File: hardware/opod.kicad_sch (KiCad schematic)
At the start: 1 part, among them U1 STM32F411CEUx

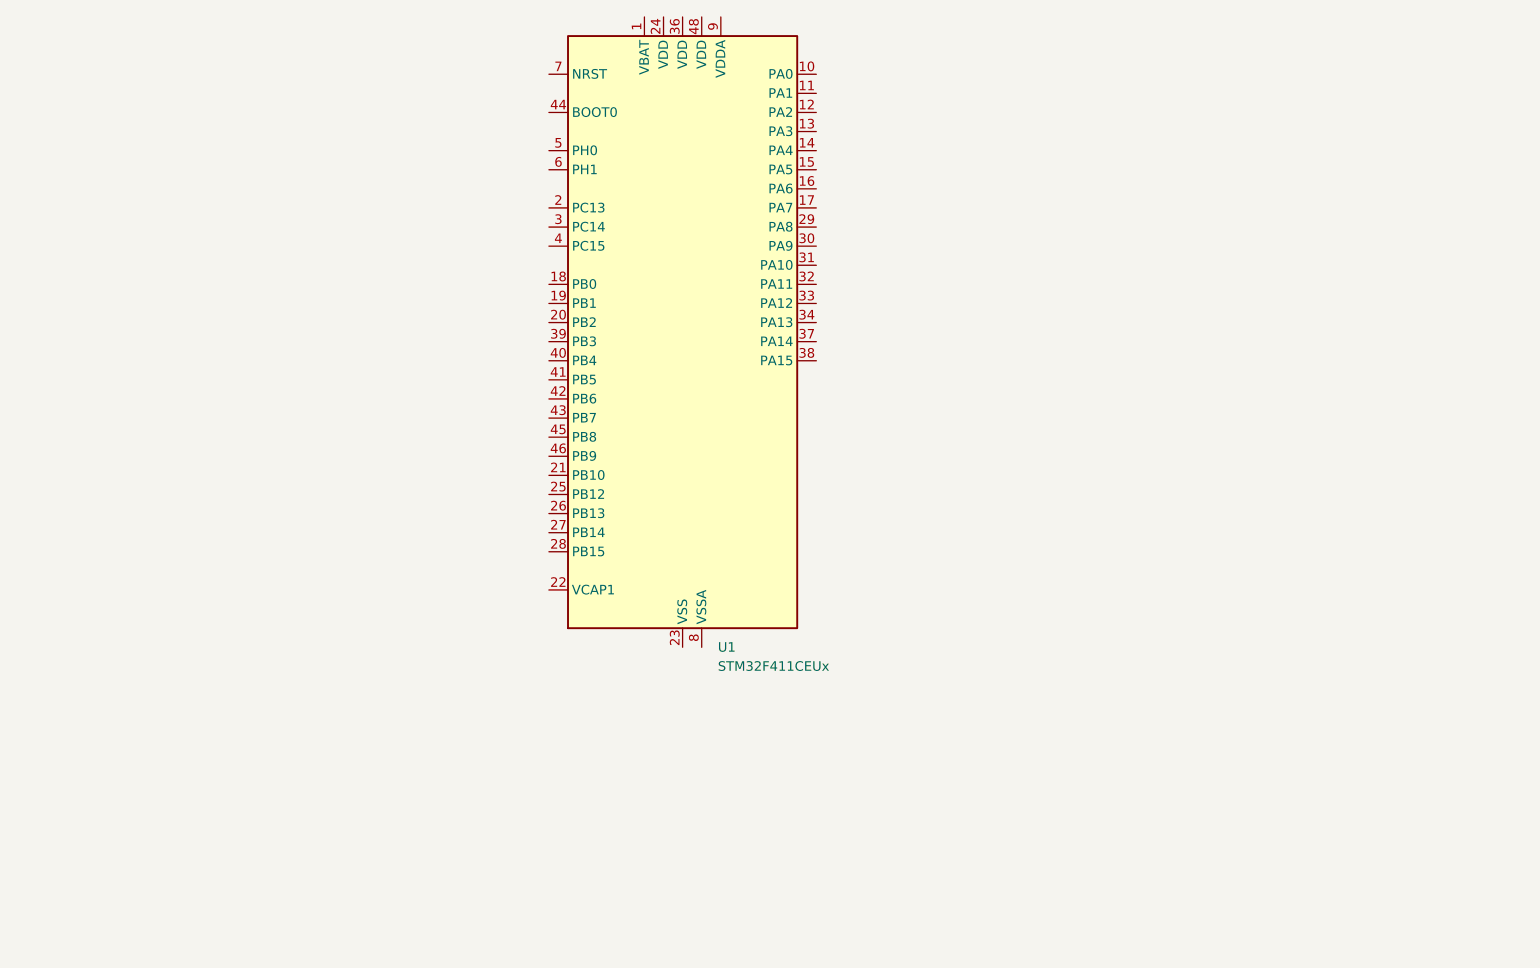
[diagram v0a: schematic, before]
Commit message: Hello, World x2
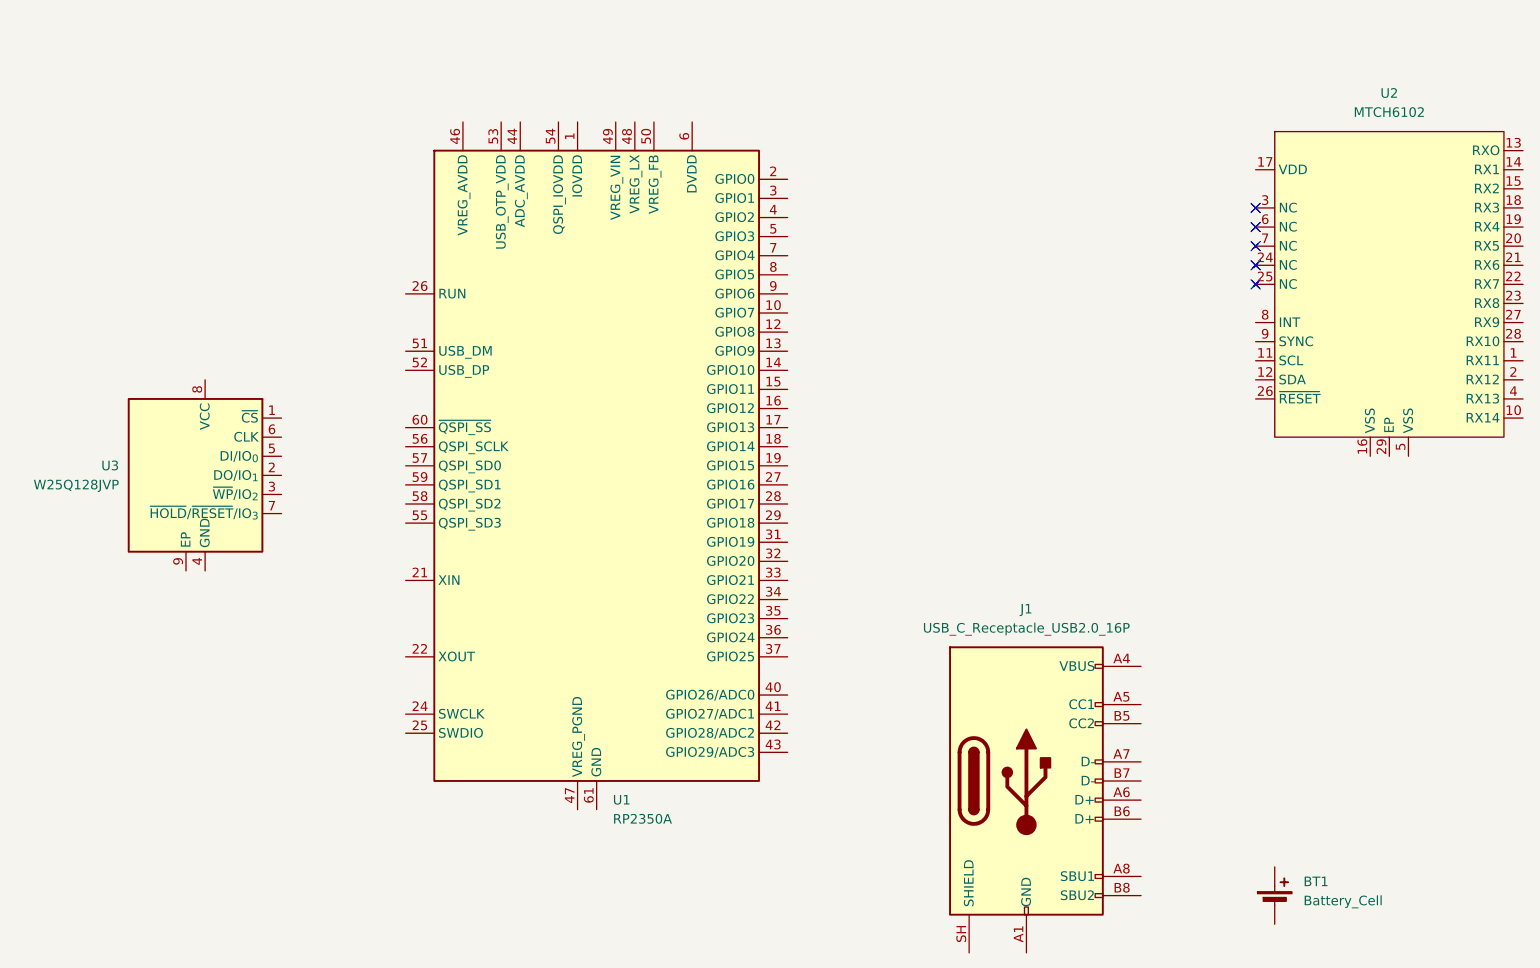
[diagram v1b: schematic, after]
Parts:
- removed U1: STM32F411CEUx, Package_DFN_QFN:QFN-48-1EP_7x7mm_P0.5mm_EP5.6x5.6mm, symbol MCU_ST_STM32F4:STM32F411CEUx
- added BT1: Battery_Cell, symbol Device:Battery_Cell
- added J1: USB_C_Receptacle_USB2.0_16P, symbol Connector:USB_C_Receptacle_USB2.0_16P
- added U1: RP2350A, Package_DFN_QFN:QFN-60-1EP_7x7mm_P0.4mm_EP3.4x3.4mm, symbol MCU_RaspberryPi:RP2350A
- added U2: MTCH6102, Package_DFN_QFN:UQFN-28-1EP_4x4mm_P0.4mm_EP2.35x2.35mm, symbol Sensor_Touch:MTCH6102-I/MV
- added U3: W25Q128JVP, Package_SON:WSON-8-1EP_6x5mm_P1.27mm_EP3.4x4.3mm, symbol Memory_Flash:W25Q128JVP
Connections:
- new net: U1.1 (IOVDD), U1.11 (IOVDD), U1.20 (IOVDD), U1.30 (IOVDD), U1.38 (IOVDD), U1.45 (IOVDD)
- new net: U1.23 (DVDD), U1.39 (DVDD), U1.6 (DVDD)
- new net: J1.A1 (GND), J1.A12 (GND), J1.B1 (GND), J1.B12 (GND)
- new net: J1.A4 (VBUS), J1.A9 (VBUS), J1.B4 (VBUS), J1.B9 (VBUS)
- no-connect marks 0 -> 5

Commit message: wiring stuff
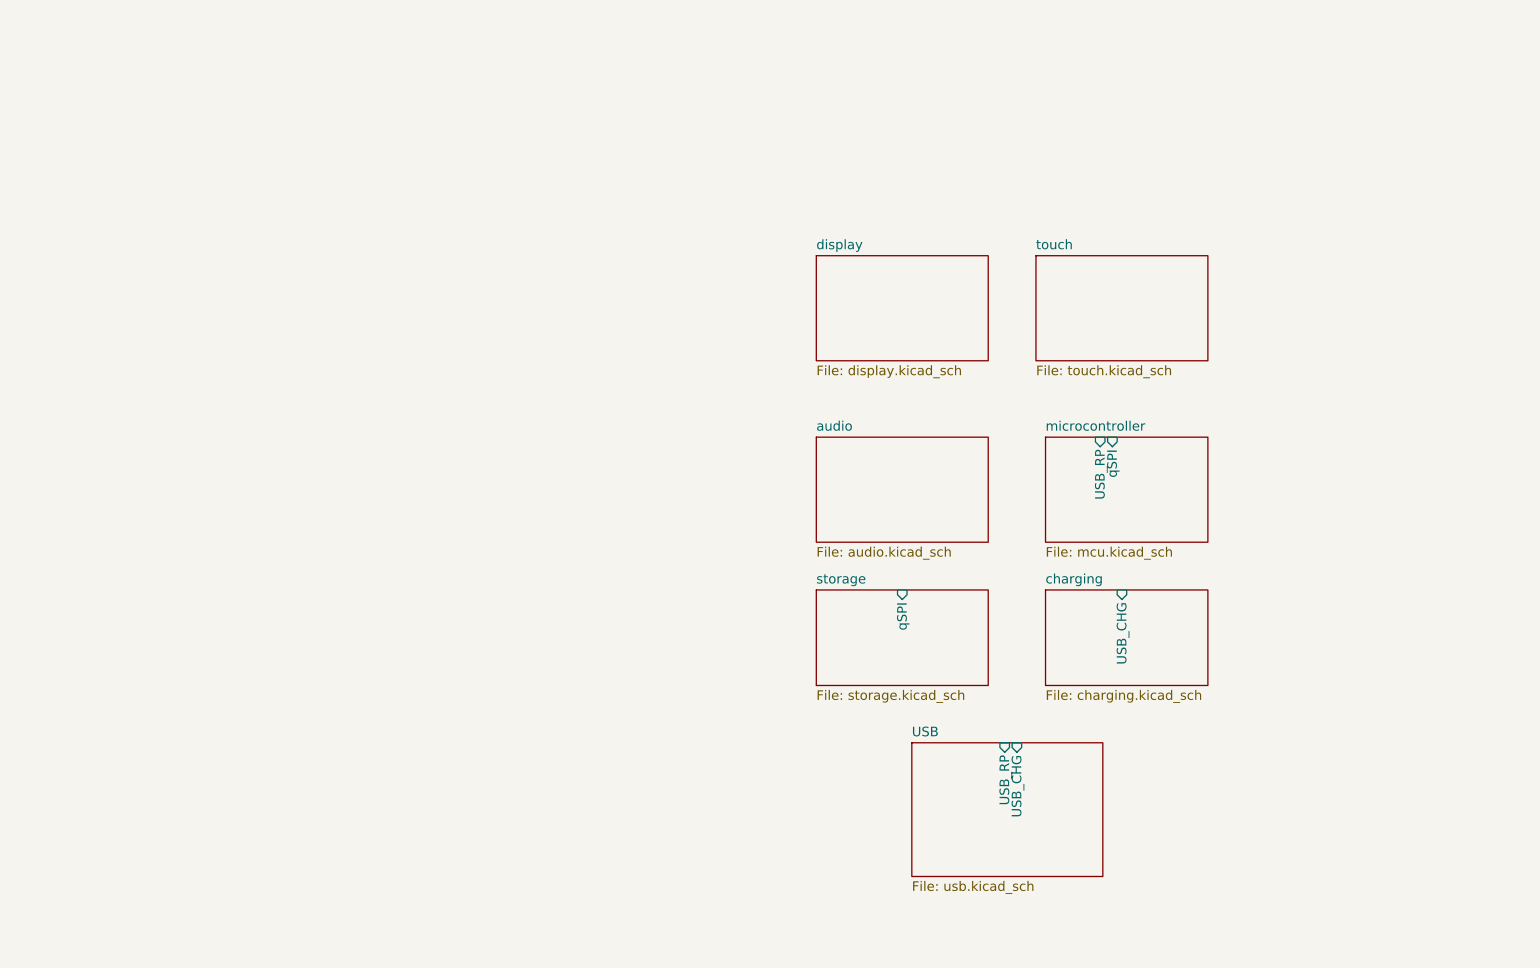
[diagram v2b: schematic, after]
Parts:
- removed BT1: Battery_Cell, symbol Device:Battery_Cell
- removed J1: USB_C_Receptacle_USB2.0_16P, symbol Connector:USB_C_Receptacle_USB2.0_16P
- removed U1: RP2350A, Package_DFN_QFN:QFN-60-1EP_7x7mm_P0.4mm_EP3.4x3.4mm, symbol MCU_RaspberryPi:RP2350A
- removed U2: MTCH6102, Package_DFN_QFN:UQFN-28-1EP_4x4mm_P0.4mm_EP2.35x2.35mm, symbol Sensor_Touch:MTCH6102-I/MV
- removed U3: W25Q128JVP, Package_SON:WSON-8-1EP_6x5mm_P1.27mm_EP3.4x4.3mm, symbol Memory_Flash:W25Q128JVP
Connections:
- no-connect marks 5 -> 0
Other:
- added sheet USB (usb.kicad_sch)
- added sheet audio (audio.kicad_sch)
- added sheet charging (charging.kicad_sch)
- added sheet display (display.kicad_sch)
- added sheet microcontroller (mcu.kicad_sch)
- added sheet storage (storage.kicad_sch)
- added sheet touch (touch.kicad_sch)
